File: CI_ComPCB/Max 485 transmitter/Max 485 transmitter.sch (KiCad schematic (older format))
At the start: 23 parts, among them IC101 74HC04D,653, IC102 SP485EEN-L_TR, J101 Conn_01x04_Male, J102 Conn_01x03_Male

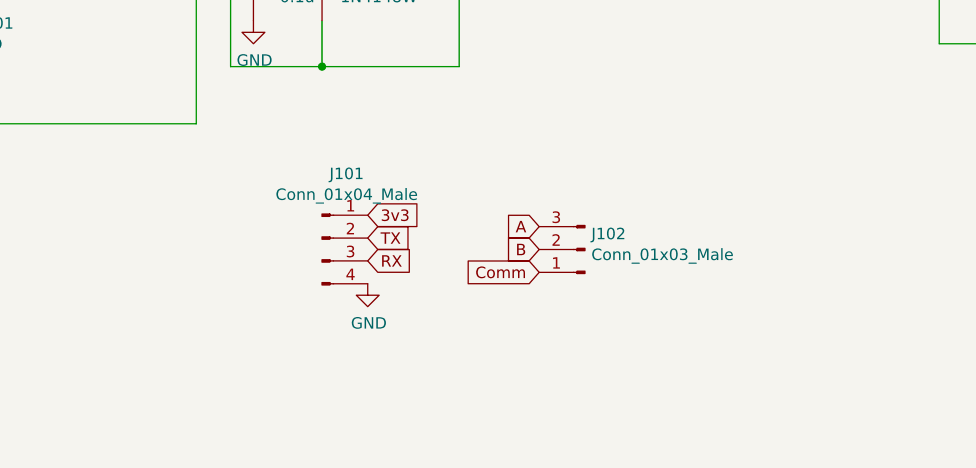
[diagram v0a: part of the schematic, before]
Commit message: Transmitter print
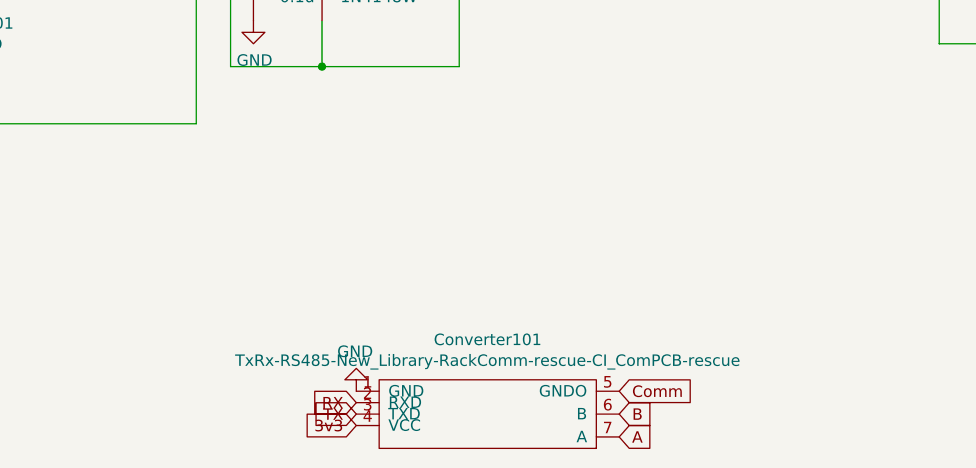
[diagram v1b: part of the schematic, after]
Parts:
- removed J101: Conn_01x04_Male, Connector_PinHeader_2.54mm:PinHeader_1x04_P2.54mm_Vertical, symbol Connector:Conn_01x04_Male
- removed J102: Conn_01x03_Male, Connector_PinHeader_2.54mm:PinHeader_1x03_P2.54mm_Vertical, symbol Connector:Conn_01x03_Male
- added Converter101: TxRx-RS485-New_Library-RackComm-rescue-CI_ComPCB-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, CI_ComPCB:TXRX-AB, symbol CI_ComPCB-rescue:TxRx-RS485-New_Library-RackComm-rescue-CI_ComPCB-rescue
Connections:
- net 3v3: now also Converter101.4 (VCC)
- net A: now also Converter101.7 (A)
- net B: now also Converter101.6 (B)
- net Comm: now also Converter101.5 (GNDO)
- net GND: now also Converter101.1 (GND)
- net RX: now also Converter101.2 (RXD)
- net TX: now also Converter101.3 (TXD)
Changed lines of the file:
@@
 Wire Wire Line
 	9500 2050 9250 2050
-$Comp
-L Connector:Conn_01x03_Male J102
-U 1 1 613641DE
-P 5550 4250
-F 0 "J102" H 5522 4182 50  0000 R CNN
-F 1 "Conn_01x03_Male" H 5522 4273 50  0000 R CNN
-F 2 "Connector_PinHeader_2.54mm:PinHeader_1x03_P2.54mm_Vertical" H 5550 4250 50  0001 C CNN
-F 3 "~" H 5550 4250 50  0001 C CNN
-	1    5550 4250
-	-1   0    0    1
-$EndComp
 Text GLabel 9600 3150 2    50   Input ~ 0
 Comm
@@
 	7700 3150 9600 3150
 Connection ~ 7700 2850
-Text GLabel 5350 4250 0    50   Input ~ 0
+Text GLabel 5700 4970 2    50   Input ~ 0
 B
-Text GLabel 5350 4150 0    50   Input ~ 0
+Text GLabel 5700 5070 2    50   Input ~ 0
 A
-Text GLabel 5350 4350 0    50   Input ~ 0
+Text GLabel 5700 4870 2    50   Input ~ 0
 Comm
 Wire Wire Line
@@
 Text GLabel 1850 1450 0    50   Input ~ 0
 3v3
-Text GLabel 4600 4100 2    50   Input ~ 0
+Text GLabel 4550 5020 0    50   Input ~ 0
 3v3
-Text GLabel 4600 4200 2    50   Input ~ 0
+Text GLabel 4550 4970 0    50   Input ~ 0
 TX
-Text GLabel 4600 4300 2    50   Input ~ 0
+Text GLabel 4550 4920 0    50   Input ~ 0
 RX
-$Comp
-L Connector:Conn_01x04_Male J101
-U 1 1 6139FDFB
-P 4400 4200
-F 0 "J101" H 4508 4481 50  0000 C CNN
-F 1 "Conn_01x04_Male" H 4508 4390 50  0000 C CNN
-F 2 "Connector_PinHeader_2.54mm:PinHeader_1x04_P2.54mm_Vertical" H 4400 4200 50  0001 C CNN
-F 3 "~" H 4400 4200 50  0001 C CNN
-	1    4400 4200
-	1    0    0    -1
-$EndComp
 $Comp
 L power:GND #PWR0107
 U 1 1 6139FE01
-P 4600 4400
-F 0 "#PWR0107" H 4600 4150 50  0001 C CNN
-F 1 "GND" H 4605 4227 50  0000 C CNN
-F 2 "" H 4600 4400 50  0001 C CNN
-F 3 "" H 4600 4400 50  0001 C CNN
-	1    4600 4400
+P 4550 4870
+F 0 "#PWR0107" H 4550 4620 50  0001 C CNN
+F 1 "GND" H 4555 4697 50  0000 C CNN
+F 2 "" H 4550 4870 50  0001 C CNN
+F 3 "" H 4550 4870 50  0001 C CNN
+	1    4550 4870
+	-1   0    0    1
+$EndComp
+$Comp
+L CI_ComPCB-rescue:TxRx-RS485-New_Library-RackComm-rescue-CI_ComPCB-rescue Converter101
+U 1 1 61323B08
+P 5150 4570
+F 0 "Converter101" H 5125 4495 50  0000 C CNN
+F 1 "TxRx-RS485-New_Library-RackComm-rescue-CI_ComPCB-rescue" H 5125 4404 50  0000 C CNN
+F 2 "CI_ComPCB:TXRX-AB" H 5150 4570 50  0001 C CNN
+F 3 "" H 5150 4570 50  0001 C CNN
+	1    5150 4570
 	1    0    0    -1
 $EndComp

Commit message: transmitter update
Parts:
- C1, C2: footprint Capacitor_SMD:C_0201_0603Metric -> Capacitor_SMD:C_0402_1005Metric
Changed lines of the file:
@@
 F 0 "C2" H 4215 3146 50  0000 L CNN
 F 1 "0.1u" H 4215 3055 50  0000 L CNN
-F 2 "Capacitor_SMD:C_0201_0603Metric" H 4138 2950 50  0001 C CNN
+F 2 "Capacitor_SMD:C_0402_1005Metric" H 4138 2950 50  0001 C CNN
 F 3 "~" H 4100 3100 50  0001 C CNN
 	1    4100 3100
@@
 F 0 "C1" H 2165 1846 50  0000 L CNN
 F 1 "0.1u" H 2165 1755 50  0000 L CNN
-F 2 "Capacitor_SMD:C_0201_0603Metric" H 2088 1650 50  0001 C CNN
+F 2 "Capacitor_SMD:C_0402_1005Metric" H 2088 1650 50  0001 C CNN
 F 3 "~" H 2050 1800 50  0001 C CNN
 	1    2050 1800
